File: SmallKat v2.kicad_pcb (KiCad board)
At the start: 4 copper layers, 104 x 56 mm, 278 parts, among them IC1 TPS562201DDCR, IC3 TPS562201DDCR, IC4 MAX34409ETE+, IC5 MAX34409ETE+, IC6 MAX34409ETE+, IC7 MAX34409ETE+, J1 Conn_01x03_Male, J10 Conn_01x03_Male, J11 Conn_01x03_Male, J12 Conn_01x03_Male, J13 Conn_01x03_Male, J14 Conn_01x03_Male, J15 Conn_01x03_Male, J16 Conn_01x03_Male, J17 Conn_01x03_Male, J19 USB_C_Receptacle, J2 Conn_01x03_Male, J21 Conn_01x05_Male, J3 Conn_01x03_Male, J4 Conn_01x03_Male, J5 Conn_01x03_Male, J6 Conn_01x03_Male, J7 Conn_01x03_Male, J8 Conn_01x03_Male, J9 Conn_01x02_Male, Q1 BUK9M120-100EX, Q10 CSD17307Q5A, Q11 CSD17307Q5A, Q12 Si7141DP, Q2 BUK9M120-100EX, Q3 MMBT3904, Q4 MMBT3904, Q7 2N3905, Q8 BUK9M120-100EX, Q9 BUK9M120-100EX, SW1 SW_SPST, SW2 SW_SPST, SW5 SW_SPST, U1 BNO055, U11 FUSB302BMPX, U12 BQ24770, U13 bq76925, U14 PCA9641, U2 LM25145RGYR, U3 ESP32-WROOM-32, U4 CP2102N-A01-GQFN24, U6 STM32L432KBUx, Y1 32.768kHz

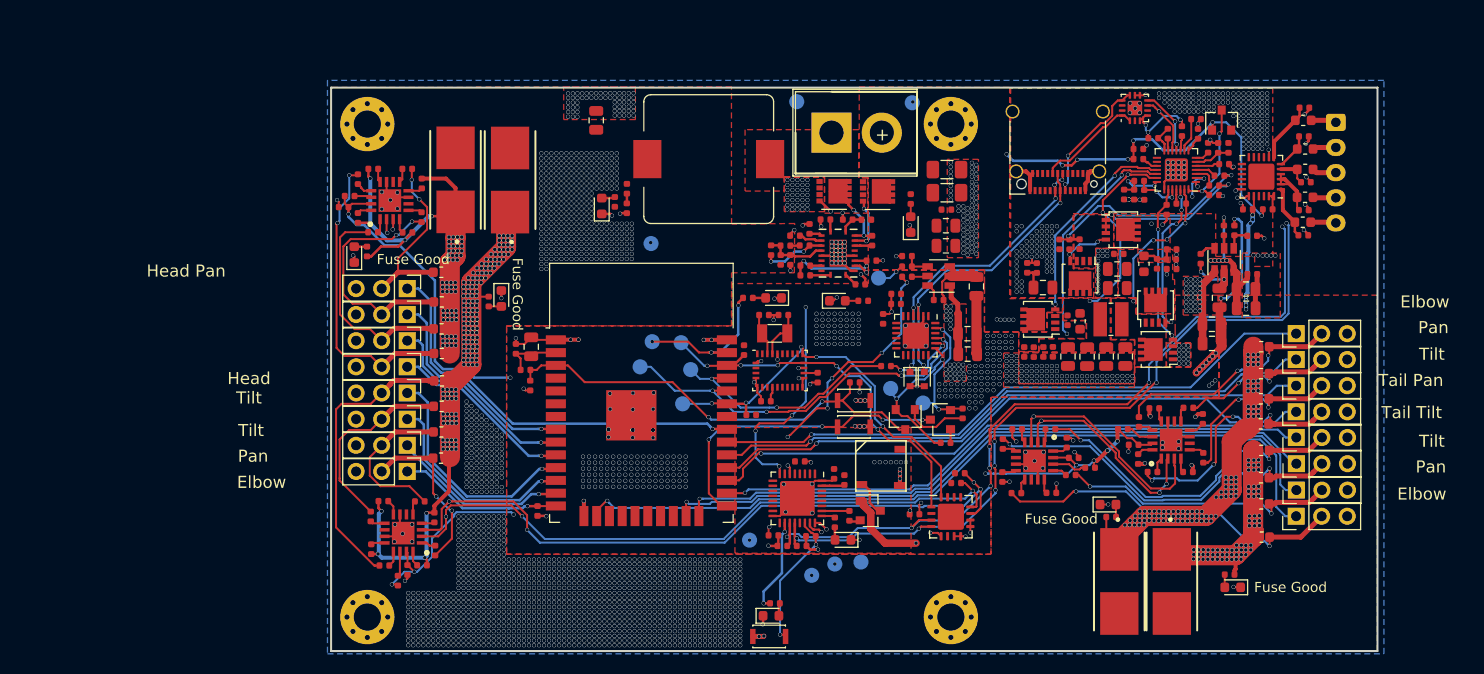
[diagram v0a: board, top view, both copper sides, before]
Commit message: Rev
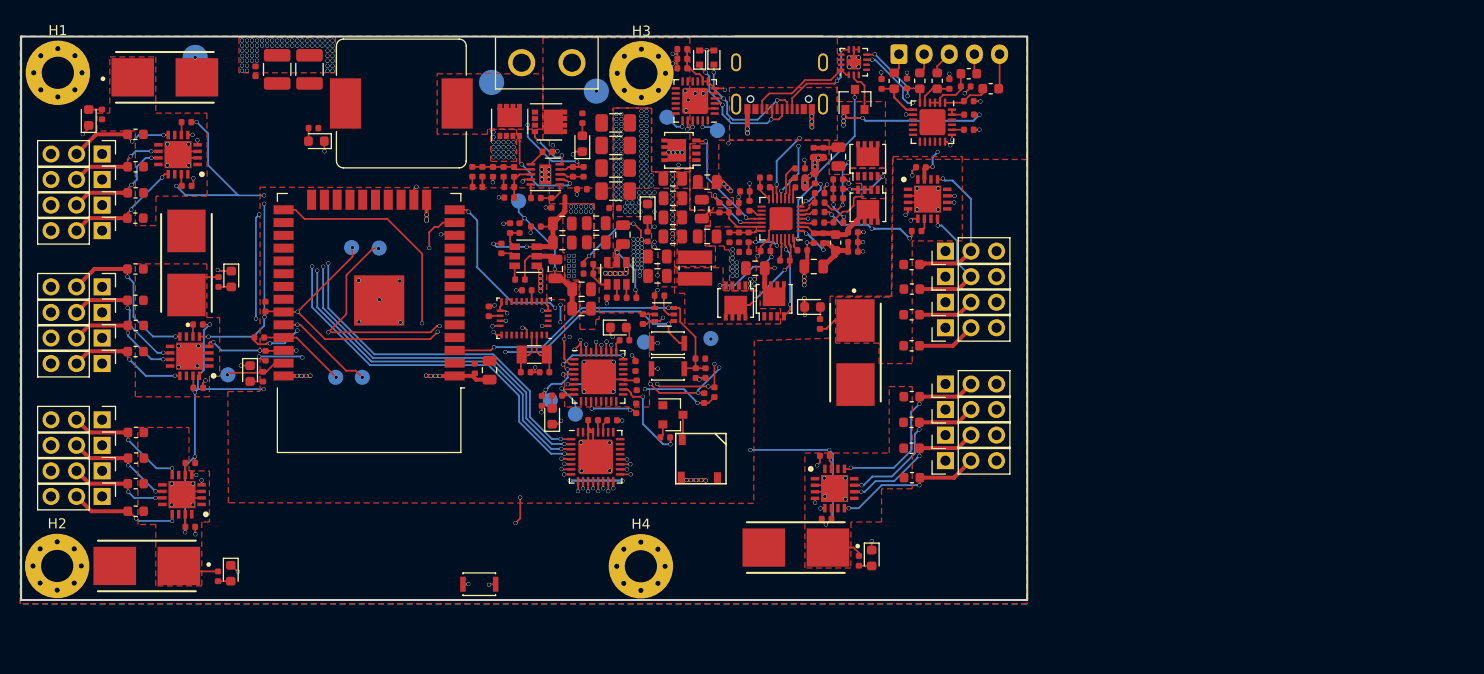
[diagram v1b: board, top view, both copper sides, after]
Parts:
- removed C45, C46, C54, C55: 0.1uF, Capacitor_SMD:C_0402_1005Metric
- removed C82: 1uF, Capacitor_SMD:C_0402_1005Metric
- removed IC4, IC5, IC6, IC7: MAX34409ETE+, MAX34409ETE+:QFN65P400X400X80-17N
- removed Q4: MMBT3904, Package_TO_SOT_SMD:SOT-23
- removed R101, R102, R103, R106, R107, R108, R109, R111, R112, R113, R114, R59, R60, R64, R65, R67, R68, R71, R72, R76, R77, R81, R82, R84, R85, R89, R90, R93, R94, R95, R96, R98: 100R, Resistor_SMD:R_0402_1005Metric
- removed R110, R83, R97: 0R, Resistor_SMD:R_0402_1005Metric
- removed R126, R127, R43: 10K, Resistor_SMD:R_0402_1005Metric
- removed U14: PCA9641, Package_DFN_QFN:UQFN-16-1EP_4x4mm_P0.65mm_EP2.6x2.6mm
- removed U2: LM25145RGYR, LM25145:LM25145RGYR
- removed U6: STM32L432KBUx, Package_DFN_QFN:QFN-32-1EP_5x5mm_P0.5mm_EP3.45x3.45mm
- added C22: C, Capacitor_SMD:C_0402_1005Metric, F.Cu at (129.2, 114.6)
- added C36: C, Capacitor_SMD:C_0402_1005Metric, F.Cu at (129.3, 116.5)
- added C38: C, Capacitor_SMD:C_0402_1005Metric, F.Cu at (125.0, 119.9)
- added C39: 47uF, Capacitor_SMD:C_1206_3216Metric, F.Cu at (127.2, 92.6)
- added C40: 47uF, Capacitor_SMD:C_1206_3216Metric, F.Cu at (127.2, 90.4)
- added C41: 1uF, Capacitor_SMD:C_0402_1005Metric, F.Cu at (91.5, 85.2)
- added C42: 0.1uF, Capacitor_SMD:C_0402_1005Metric, F.Cu at (148.0, 123.5)
- added C43: 0.1uF, Capacitor_SMD:C_0402_1005Metric, F.Cu at (157.6, 94.8)
- added D9: LED, LED_SMD:LED_0603_1608Metric, F.Cu at (146.8, 108.7)
- added F5: Fuse, 01550900M:0154.250DR, F.Cu at (151.1, 113.2)
- added IC8: TPS40192DRCT-TPS40192DRCT, Package_SON:VSON-10-1EP_3x3mm_P0.5mm_EP1.2x2mm, F.Cu at (120.2, 95.5)
- added J18: Conn_01x03_Male, Connector_PinHeader_2.54mm:PinHeader_1x03_P2.54mm_Vertical, F.Cu at (160.0, 110.7)
- added J20: Conn_01x03_Male, Connector_PinHeader_2.54mm:PinHeader_1x03_P2.54mm_Vertical, F.Cu at (160.0, 105.7)
- added J22: Conn_01x03_Male, Connector_PinHeader_2.54mm:PinHeader_1x03_P2.54mm_Vertical, F.Cu at (160.0, 108.2)
- added J23: Conn_01x03_Male, Connector_PinHeader_2.54mm:PinHeader_1x03_P2.54mm_Vertical, F.Cu at (160.0, 103.1)
- added PS1: PAC1934T-I_JQ, PAC1934T-I_JQ:QFN65P400X400X55-17N-D, F.Cu at (83.7, 93.5)
- added PS2: PAC1934T-I_JQ, PAC1934T-I_JQ:QFN65P400X400X55-17N-D, F.Cu at (84.9, 113.6)
- added PS3: PAC1934T-I_JQ, PAC1934T-I_JQ:QFN65P400X400X55-17N-D, F.Cu at (84.1, 127.3)
- added PS4: PAC1934T-I_JQ, PAC1934T-I_JQ:QFN65P400X400X55-17N-D, F.Cu at (149.0, 126.7)
- added PS5: PAC1934T-I_JQ, PAC1934T-I_JQ:QFN65P400X400X55-17N-D, F.Cu at (158.3, 98.0)
- added R128: 20K, Resistor_SMD:R_0402_1005Metric, F.Cu at (147.6, 110.4)
- added R32: 3.3K, Resistor_SMD:R_0402_1005Metric, F.Cu at (126.9, 119.9)
- added R33: 0.01R, Resistor_SMD:R_0603_1608Metric, F.Cu at (156.7, 112.5)
- added R34: 0.01R, Resistor_SMD:R_0603_1608Metric, F.Cu at (156.7, 106.9)
- added R35: 0.01R, Resistor_SMD:R_0603_1608Metric, F.Cu at (156.7, 109.4)
- added R36: 0.01R, Resistor_SMD:R_0603_1608Metric, F.Cu at (156.7, 104.5)
- added R39: 0R, Resistor_SMD:R_0402_1005Metric, F.Cu at (148.2, 129.7)
- added R40: 0R, Resistor_SMD:R_0402_1005Metric, F.Cu at (157.2, 101.1)
- added TP8: TestPoint, TestPoint:TestPoint_Pad_D1.5mm, B.Cu at (120.8, 118.0)
- added U5: LPC824M201JHI33, Package_DFN_QFN:QFN-32-1EP_5x5mm_P0.5mm_EP3.45x3.45mm, F.Cu at (125.6, 115.6)
- added U7: TLC5947RHB, Package_DFN_QFN:QFN-32-1EP_5x5mm_P0.5mm_EP3.45x3.45mm, F.Cu at (125.3, 123.6)
- C10: value 10uF -> 1000pF; footprint Capacitor_SMD:C_1206_3216Metric -> Capacitor_SMD:C_0402_1005Metric
- C11: value 10uF -> 100pF; footprint Capacitor_SMD:C_1206_3216Metric -> Capacitor_SMD:C_0402_1005Metric
- C12: value 2.2uF -> 10nF
- C13: value 0.1uF -> 1uF
- C14: value 6.8nF -> 4.7uF
- C15: value 0.1uF -> 470nF
- C16: value 5.6nF -> 10uF; footprint Capacitor_SMD:C_0402_1005Metric -> Capacitor_SMD:C_1206_3216Metric
- C18: value 1pF -> 10uF; footprint Capacitor_SMD:C_0402_1005Metric -> Capacitor_SMD:C_1206_3216Metric
- C19: value 330pF -> 100uF; footprint Capacitor_SMD:C_0402_1005Metric -> Capacitor_SMD:C_1210_3225Metric
- C21: value 10uF -> 100uF; footprint Capacitor_SMD:C_0805_2012Metric -> Capacitor_SMD:C_1210_3225Metric
- C69, C74: footprint Capacitor_SMD:C_0402_1005Metric -> Capacitor_SMD:C_0805_2012Metric
- H1, H2, H3, H4: footprint MountingHole:MountingHole_2.7mm_M2.5_Pad_Via -> MountingHole:MountingHole_3.2mm_M3_Pad_Via
- J19: footprint Connector_USB:USB_C_Receptacle_Amphenol_12401610E4-2A_CircularHoles -> C167321:C167321
- J9: footprint SmallKat ESP32:SHDR2W320P716_1X2_1574X813X1588P -> XT30PB:XT30PB
- Q3: value MMBT3904 -> MBT3904DW1; footprint Package_TO_SOT_SMD:SOT-23 -> Package_TO_SOT_SMD:SOT-363_SC-70-6
- R12: value 20K -> 2.18k
- R123: footprint Resistor_SMD:R_0603_1608Metric -> Resistor_SMD:R_0805_2012Metric
- R13: value 2.1R -> 20k
- R14: value 10K -> 2.61k
- R15: value 10K -> 4.22k
- R16: value 20K -> 3.9k
- R17: value 20K -> 100k
- R18: value 634R -> 100k
- R19: value 2.49K -> 100k
- R20: value 18K -> 1K
- R29: value 2.74K -> 0R
- R30: value 29.4R -> 0R
- TP4, TP6, TP7: footprint TestPoint:TestPoint_Pad_D1.5mm -> TestPoint:TestPoint_Pad_D2.5mm
- moved J2 119.1 mm to (76.2, 119.9), turned to 270 degrees
- moved J8 118.8 mm to (76.2, 127.5), turned to 270 degrees
- moved J4 118.8 mm to (76.2, 122.4), turned to 270 degrees
- moved J6 118.7 mm to (76.2, 125.0), turned to 270 degrees
- moved R62 112.4 mm to (79.6, 121.1), turned to 0 degrees
- moved R80 112.0 mm to (79.5, 129.0), turned to 0 degrees
- moved R70 111.9 mm to (79.6, 123.7), turned to 0 degrees
- moved R75 111.8 mm to (79.5, 126.2), turned to 0 degrees
- moved H1 103.9 mm to (71.8, 85.4)
- moved F3 101.9 mm to (80.6, 134.4), turned to 180 degrees
- moved R78 100.5 mm to (87.7, 135.4), turned to 270 degrees
- moved D25 99.6 mm to (89.0, 135.1), turned to 270 degrees
- moved C52 88.1 mm to (85.0, 130.5)
- moved R2 73.8 mm to (116.7, 100.8), turned to 270 degrees
- moved R28 71.8 mm to (115.9, 102.9)
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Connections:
- C10 pad 1: +BATT -> +6V
- C10 pad 2: GND -> Net-(C10-Pad2)
- C11 pad 1: +BATT -> Net-(C11-Pad1)
- C11 pad 2: GND -> Net-(C11-Pad2)
- C12 pad 1: Net-(C12-Pad1) -> Net-(C11-Pad1)
- C12 pad 2: GND -> Net-(C12-Pad2)
- C13 pad 1: Net-(C13-Pad1) -> +BATT
- C16 pad 1: Net-(C16-Pad1) -> +BATT
- C16 pad 2: Net-(C16-Pad2) -> GND
- C18 pad 1: Net-(C18-Pad1) -> +BATT
- C18 pad 2: Net-(C16-Pad2) -> GND
- C19 pad 1: Net-(C19-Pad1) -> +6V
- C37 pad 1: +3.3VA -> +3V3
- Q3 pad 1: Net-(Q3-Pad1) -> /MainBoard/ESP32Module/RTS
- Q3 pad 2: /MainBoard/ESP32Module/RTS -> Net-(Q3-Pad2)
- Q3 pad 3: /MainBoard/ESP32Module/EN -> /MainBoard/ESP32Module/DTR
- R12 pad 1: +6V -> Net-(C11-Pad2)
- R12 pad 2: Net-(D4-Pad2) -> GND
- R13 pad 1: +BATT -> +6V
- R13 pad 2: Net-(C13-Pad1) -> Net-(C11-Pad2)
- R14 pad 1: Net-(R14-Pad1) -> Net-(C11-Pad2)
- R14 pad 2: /MainBoard/6VEN -> Net-(C10-Pad2)
- R15 pad 1: Net-(R15-Pad1) -> Net-(C12-Pad2)
- R15 pad 2: GND -> Net-(C11-Pad2)
- R16 pad 1: Net-(R16-Pad1) -> Net-(C11-Pad1)
- R16 pad 2: Net-(C12-Pad1) -> GND
- R17 pad 1: Net-(R17-Pad1) -> /MainBoard/6VEN
- R17 pad 2: Net-(C12-Pad1) -> Net-(IC8-Pad1)
- R18 pad 1: Net-(C15-Pad1) -> Net-(C14-Pad1)
- R19 pad 1: Net-(C18-Pad1) -> Net-(C15-Pad1)
- R19 pad 2: Net-(C16-Pad1) -> Net-(C15-Pad2)
- R20 pad 2: Net-(C18-Pad1) -> Net-(D4-Pad2)
- R21 pad 1: /MainBoard/SERVO0 -> /MainBoard/NRST
- R25 pad 1: Net-(Q3-Pad1) -> Net-(Q3-Pad2)
- R26 pad 1: Net-(Q4-Pad1) -> Net-(Q3-Pad5)
- R29 pad 1: Net-(C18-Pad1) -> Net-(PS2-Pad6)
- R29 pad 2: GND -> +3V3
- R30 pad 1: +6V -> Net-(PS3-Pad6)
- R30 pad 2: Net-(C19-Pad1) -> +3V3
- R66 pad 1: +3V3 -> Net-(PS1-Pad6)
- R66 pad 2: Net-(IC4-Pad14) -> +3V3
- TP4 pad 1: +BATT -> +6V
- TP6 pad 1: GND -> +BATT
- TP7 pad 1: +6V -> GND
- U3 pad 10: /MainBoard/SERVO4 -> (no net)
- U3 pad 11: /MainBoard/SERVO3 -> (no net)
- U3 pad 12: /MainBoard/SERVO2 -> /MainBoard/TX1
- U3 pad 13: /MainBoard/SERVO1 -> /MainBoard/RX1
- U3 pad 14: /MainBoard/SERVO0 -> /MainBoard/NRST
- U3 pad 16: /MainBoard/SERVO8 -> /MainBoard/TALKALLOWED
- U3 pad 23: /MainBoard/SERVO9 -> (no net)
- U3 pad 24: /MainBoard/SERVO10 -> (no net)
- U3 pad 26: /MainBoard/SERVO11 -> (no net)
- U3 pad 27: /MainBoard/SERVO12 -> (no net)
- U3 pad 28: /MainBoard/SERVO13 -> (no net)
- U3 pad 29: /MainBoard/SERVO14 -> (no net)
- U3 pad 30: /MainBoard/SERVO15 -> (no net)
- U3 pad 31: /MainBoard/SERVO7 -> (no net)
- U3 pad 8: /MainBoard/SERVO6 -> (no net)
- U3 pad 9: /MainBoard/SERVO5 -> (no net)
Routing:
- net /MainBoard/_SCL: track 131.4 -> 0.00 mm, vias 6 -> 0
- net /MainBoard/_SDA: track 128.6 -> 0.00 mm, vias 7 -> 0
- net /MainBoard/SCL: track 38.7 -> 154.9 mm, vias 5 -> 14
- net /MainBoard/SDA: track 39.6 -> 155.3 mm, vias 5 -> 13
- net /MainBoard/Servos/6V4: track 111.9 -> 3.60 mm, vias 104 -> 0
- net /MainBoard/Servos/6V1: track 104.9 -> 0.00 mm, vias 164 -> 0
- net /MainBoard/Servos/6V3: track 90.1 -> 4.12 mm, vias 71 -> 0
- net /MainBoard/SERVO0: track 16.4 -> 98.7 mm, vias 1 -> 2
- net /MainBoard/Servos/6V2: track 66.7 -> 3.92 mm, vias 64 -> 0
- net Net-(R24-Pad2): track 7.54 -> 62.5 mm, vias 2 -> 5
- net /MainBoard/SERVO1: track 17.8 -> 61.6 mm, vias 1 -> 2
- net /MainBoard/SERVO19: track 0.00 -> 43.4 mm, vias 0 -> 1
- net +3.3VA: track 63.7 -> 21.7 mm, vias 19 -> 4
- net /MainBoard/SERVO18: track 0.00 -> 41.2 mm, vias 0 -> 1
- net /MainBoard/SERVO2: track 20.9 -> 60.8 mm, vias 1 -> 2
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- added copper zone on F.Cu, net /MainBoard/Servos/6V1
- added copper zone on F.Cu, net /MainBoard/Servos/6V2
- added copper zone on F.Cu, net /MainBoard/Servos/6V3
- added copper zone on F.Cu, net /MainBoard/Servos/6V4
- added copper zone on F.Cu, net /MainBoard/Servos/6V5
- removed copper zone on In1.Cu, net +3.3VA
- removed copper zone on In1.Cu, net GND
- removed copper zone on F.Cu, net Net-(C50-Pad2)
- removed copper zone on F.Cu, net Net-(C57-Pad1)
- removed copper zone on In1.Cu, net VBUS
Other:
- board size 104 x 56 mm -> 100 x 56 mm
- net class Default: clearance 0.127 -> 0.1778; trace_width 0.127 -> 0.1778
- rule trace_clearance: 0.127 -> 0.1778
- board text removed: "+"
- board text removed: "BATT+"
- board text removed: "Elbow"
- board text removed: "Fuse Good"
- board text removed: "Head Pan"
- board text removed: "Head Tilt"
- board text removed: "Pan"
- board text removed: "Tail Pan"
- board text removed: "Tail Tilt"
- board text removed: "Tilt"
